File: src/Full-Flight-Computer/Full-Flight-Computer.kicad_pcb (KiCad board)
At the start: 4 copper layers, 74.7 x 30.2 mm, 90 parts, among them J1 Jumper_NO, P1 0530470610, P2 B2B-PH-K-SLFSN_JST, P3 1984659, P4 1546551-4, P5 1984659, P6 USB, Q1 QS5U17TR, Q10 2N7002W-7-F, Q2 QS5U17TR, Q3 QS5U17TR, Q4 QS5U17TR, Q5 2N7002W-7-F, Q6 2N7002W-7-F, Q7 2N7002W-7-F, Q8 2N7002W-7-F, Q9 2N7002W-7-F, U1 STM32H750VBTx, U2 AP7370-33Y-13, U3 BMI323, U4 BMM150, U5 BMP390, U6 H3LIS100DLTR, U7 SST25VF040B-50-4I-S2AE-T, U8 CP2102-GMR(QFN28), Y1 ECS-240-18-33-JGN-TR

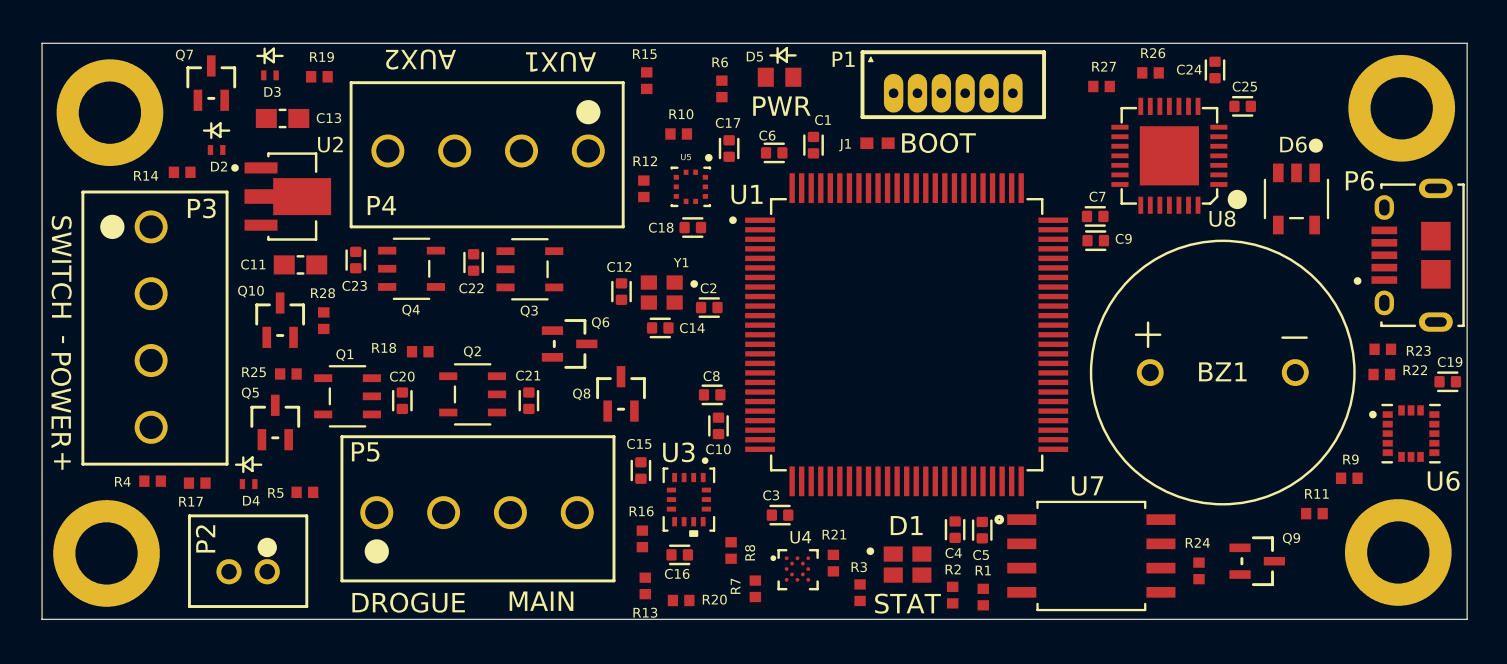
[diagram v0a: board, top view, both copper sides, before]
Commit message: completed initial layout
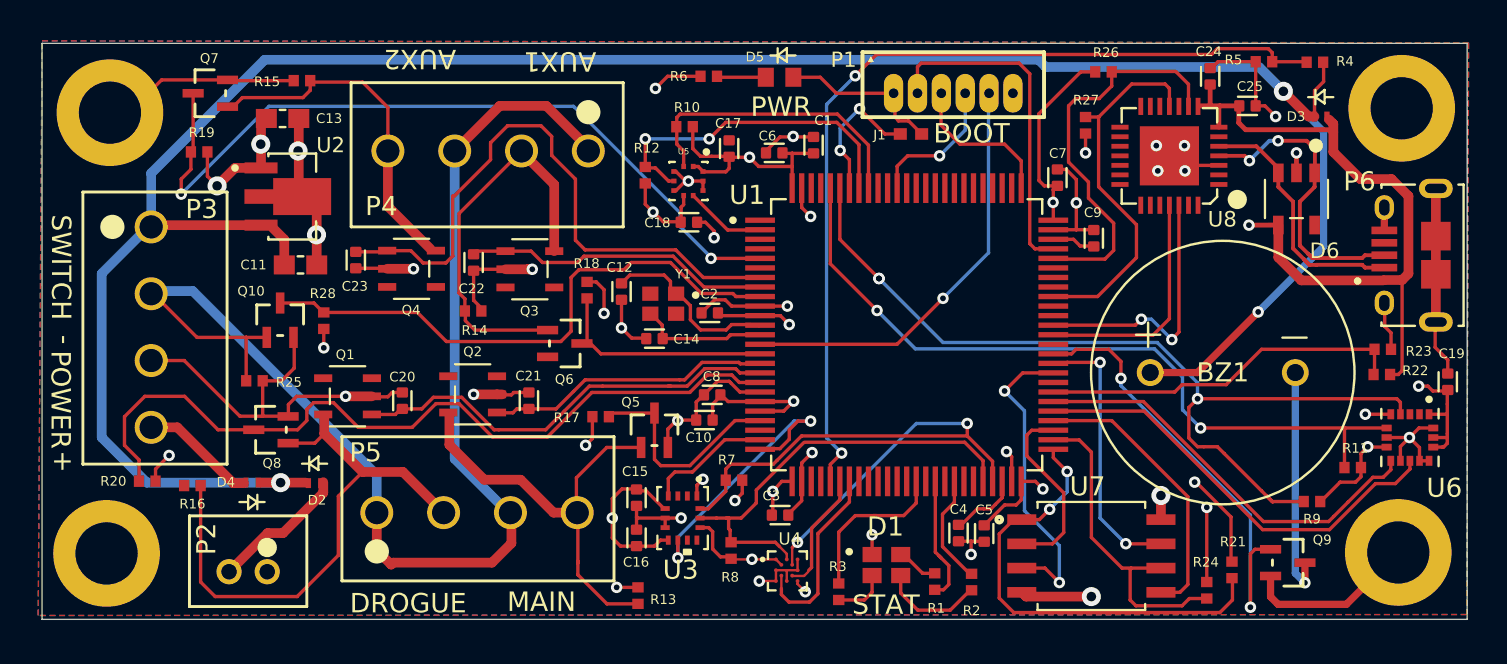
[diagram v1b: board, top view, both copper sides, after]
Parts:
- moved R4 64.7 mm to (159.7, 72.4), turned to 180 degrees
- moved D3 55.1 mm to (160.0, 75.3)
- moved R5 55.1 mm to (157.0, 72.4)
- moved R20 28.7 mm to (98.5, 94.4)
- moved R16 23.7 mm to (100.9, 94.6), turned to 0 degrees
- moved R17 21.4 mm to (122.3, 91.0)
- moved R21 20.9 mm to (155.3, 99.0)
- moved Q5 19.9 mm to (125.1, 91.7)
- moved Q8 18.4 mm to (105.0, 91.7), turned to 90 degrees
- moved D2 18.2 mm to (107.3, 94.5)
- moved R15 18.1 mm to (106.6, 73.4), turned to 0 degrees
- moved R14 16.9 mm to (115.6, 85.5), turned to 180 degrees
- moved R18 9.31 mm to (121.6, 84.4), turned to 90 degrees
- moved R19 7.43 mm to (101.2, 77.1)
- moved R7 5.80 mm to (129.3, 94.3), turned to 0 degrees
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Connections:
- U1 pad 15: unconnected-(U1-PC0-Pad15) -> ~{AUX1_CONT}
- U1 pad 16: unconnected-(U1-PC1-Pad16) -> MAIN
- U1 pad 17: IMU_INT1 -> DROGUE
- U1 pad 18: unconnected-(U1-PC3_C-Pad18) -> ~{DROGUE_CONT}
- U1 pad 22: unconnected-(U1-PA0-Pad22) -> ~{MAIN_CONT}
- U1 pad 24: IMU_INT2 -> IMU_INT1
- U1 pad 25: unconnected-(U1-PA3-Pad25) -> IMU_INT2
- U1 pad 3: ~{MAIN_CONT} -> unconnected-(U1-PE4-Pad3)
- U1 pad 31: unconnected-(U1-PA7-Pad31) -> MAG_DRDY
- U1 pad 32: unconnected-(U1-PC4-Pad32) -> MAG_INT
- U1 pad 34: HG_ACC_INT1 -> unconnected-(U1-PB0-Pad34)
- U1 pad 35: HG_ACC_INT2 -> unconnected-(U1-PB1-Pad35)
- U1 pad 36: MAG_DRDY -> unconnected-(U1-PB2-Pad36)
- U1 pad 37: MAG_INT -> unconnected-(U1-PE7-Pad37)
- U1 pad 39: unconnected-(U1-PE9-Pad39) -> STATUS_R
- U1 pad 41: unconnected-(U1-PE11-Pad41) -> STATUS_B
- U1 pad 42: AUX1 -> unconnected-(U1-PE12-Pad42)
- U1 pad 43: AUX2 -> STATUS_G
- U1 pad 44: ~{AUX1_CONT} -> unconnected-(U1-PE14-Pad44)
- U1 pad 45: ~{AUX2_CONT} -> unconnected-(U1-PE15-Pad45)
- U1 pad 5: unconnected-(U1-PE6-Pad5) -> ~{AUX2_CONT}
- U1 pad 55: unconnected-(U1-PD8-Pad55) -> HG_ACC_INT1
- U1 pad 56: USB_DETECT -> HG_ACC_INT2
- U1 pad 57: unconnected-(U1-PD10-Pad57) -> USB_DETECT
- U1 pad 68: STATUS_B -> unconnected-(U1-PA9-Pad68)
- U1 pad 69: STATUS_G -> unconnected-(U1-PA10-Pad69)
- U1 pad 7: DROGUE -> AUX2
- U1 pad 70: STATUS_R -> unconnected-(U1-PA11-Pad70)
- U1 pad 8: ~{DROGUE_CONT} -> AUX1
- U1 pad 87: MAIN -> unconnected-(U1-PD6-Pad87)
- U1 pad 88: ~{SWITCH} -> unconnected-(U1-PD7-Pad88)
- U1 pad 9: unconnected-(U1-PC15-Pad9) -> ~{SWITCH}
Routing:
- net Earth: track 0.00 -> 140.1 mm, vias 0 -> 33
- net VIN: track 0.00 -> 123.9 mm, vias 0 -> 3
- net 3.3V: track 0.00 -> 102.7 mm, vias 0 -> 22
- net VIN_SW: track 0.00 -> 67.4 mm
- net VBAT_SENSE: track 0.00 -> 47.2 mm, vias 0 -> 2
- net HG_ACC_SCL: track 0.00 -> 46.8 mm, vias 0 -> 3
- net ~{DROGUE_CONT}: track 0.00 -> 42.4 mm
- net ~{AUX2_CONT}: track 0.00 -> 41.6 mm, vias 0 -> 2
- net HG_ACC_SDA: track 0.00 -> 39.8 mm, vias 0 -> 2
- net 5V: track 0.00 -> 37.1 mm, vias 0 -> 1
- net SDA: track 0.00 -> 32.6 mm, vias 0 -> 2
- net AUX2: track 0.00 -> 31.9 mm
- net ~{SWITCH}: track 0.00 -> 29.8 mm
- net Net-(P5A-6): track 0.00 -> 29.3 mm
- net ~{FLASH_SS}: track 0.00 -> 24.3 mm, vias 0 -> 2
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- added copper zone on In2.Cu, net 3.3V
- added copper zone on B.Cu, net Earth
- added copper zone on F.Cu, net Earth
- added copper zone on In1.Cu, net Earth

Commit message: resolved all DRC errors
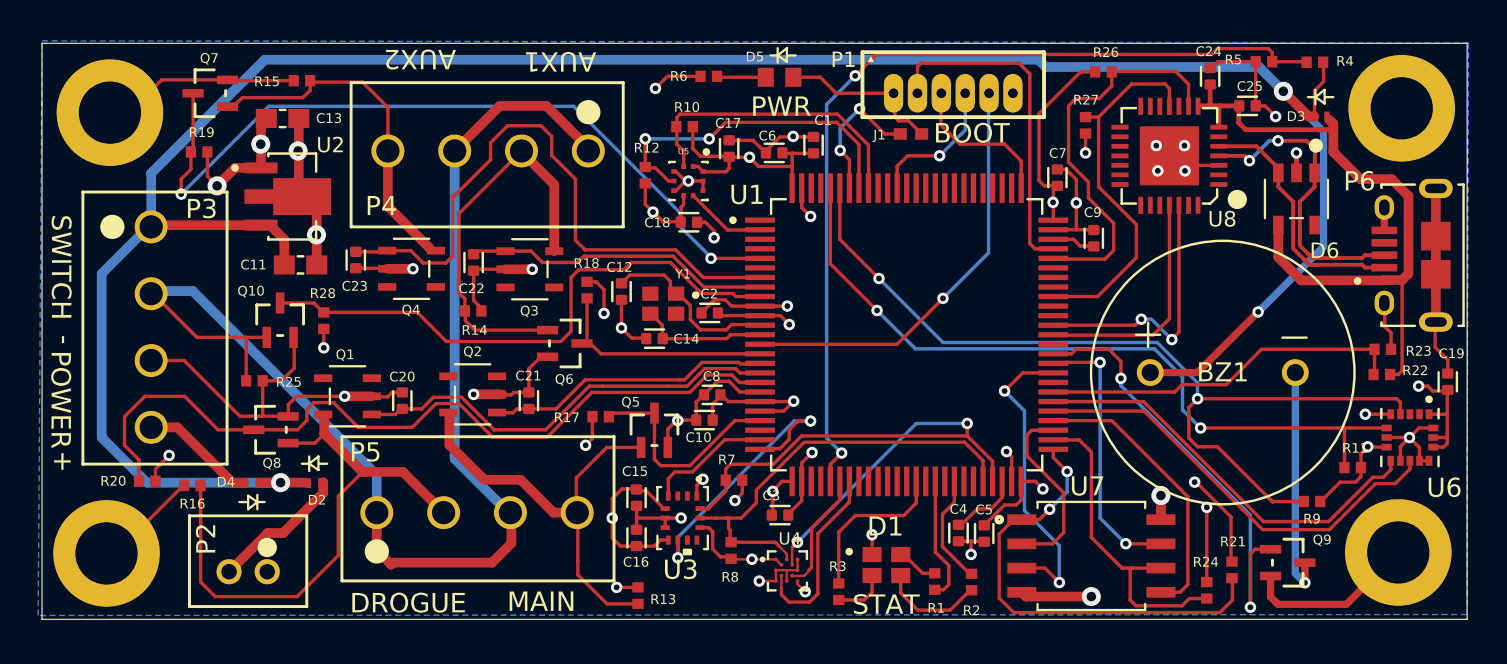
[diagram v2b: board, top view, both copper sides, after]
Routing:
- net Earth: track 140.1 -> 146.5 mm
- net 5V: track 37.1 -> 35.6 mm, vias 1 -> 0
- net HG_ACC_SCL: vias 3 -> 2
- removed copper zone on F.Cu, net Earth
